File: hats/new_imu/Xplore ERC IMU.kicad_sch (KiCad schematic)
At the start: 42 parts, among them J1 5025850670, J2 5025850670, U1 LIS3MDL, U2 BMI088, U3 LT3960JMSE-PBF, U4 AMS1117-3.3, U5 D5V0H1B2LP-7B

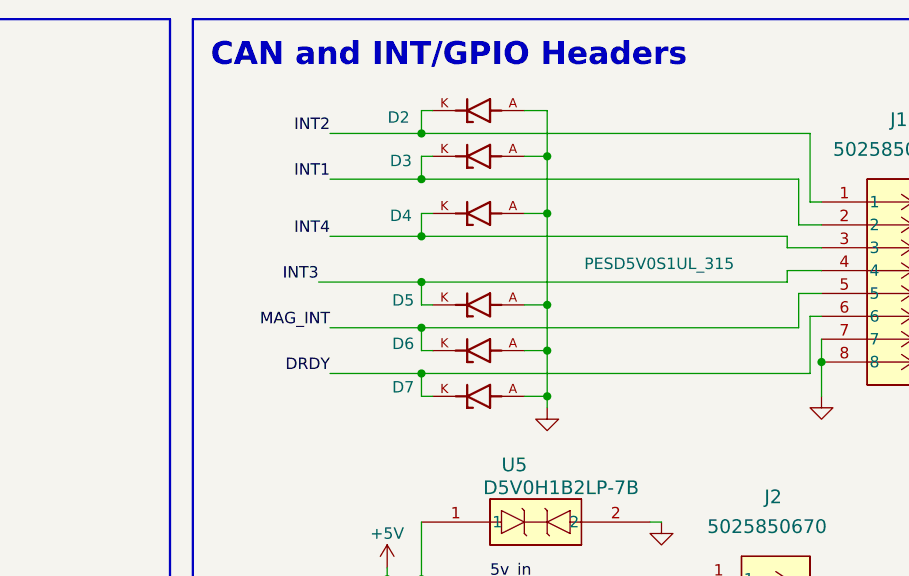
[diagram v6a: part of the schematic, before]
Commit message: Pedro review
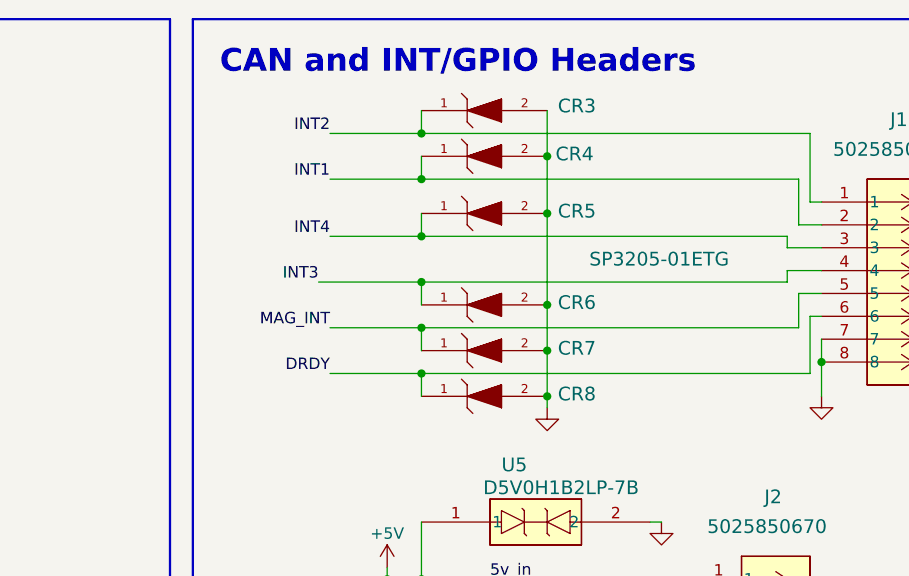
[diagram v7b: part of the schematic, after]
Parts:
- removed D2, D3, D4, D5, D6, D7: PESD5V0S1UL_315, footprints:DIO_PESD5V0S1UL_315, symbol PESD5V0S1UL_315:PESD5V0S1UL_315
- added CR3, CR4, CR5, CR6, CR7, CR8: SP3205-01ETG, footprints:SDO_SOD882_LTF, symbol SP3205_01ETG:SP3205-01ETG
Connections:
- net DRDY: now also CR8.1
- net GND: now also CR3.2, CR4.2, CR5.2, CR6.2, CR7.2, CR8.2
- net INT1: now also CR4.1
- net INT2: now also CR3.1
- net INT3: now also CR6.1
- net INT4: now also CR5.1
- net MAG_INT: now also CR7.1

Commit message: changed R size
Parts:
- R1, R3, R4, R7: footprint Resistor_SMD:R_0402_1005Metric -> Resistor_SMD:R_0603_1608Metric
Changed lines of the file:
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@@
 			)
 		)
-		(property "Footprint" "Resistor_SMD:R_0402_1005Metric"
+		(property "Footprint" "Resistor_SMD:R_0603_1608Metric"
 			(at 139.7 130.81 0)
 			(effects
@@
 			)
 		)
-		(property "Footprint" "Resistor_SMD:R_0402_1005Metric"
+		(property "Footprint" "Resistor_SMD:R_0603_1608Metric"
 			(at 139.7 156.21 0)
 			(effects
@@
 			)
 		)
-		(property "Footprint" "Resistor_SMD:R_0402_1005Metric"
+		(property "Footprint" "Resistor_SMD:R_0603_1608Metric"
 			(at 139.7 168.91 0)
 			(effects
@@
 			)
 		)
-		(property "Footprint" "Resistor_SMD:R_0402_1005Metric"
+		(property "Footprint" "Resistor_SMD:R_0603_1608Metric"
 			(at 139.7 143.51 0)
 			(effects
